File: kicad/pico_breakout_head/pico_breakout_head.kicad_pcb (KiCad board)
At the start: 2 copper layers, 39 x 66 mm, 19 parts, among them J1 HDR F 2.54MM 20-pin VERT, J2 HDR F 2.54MM 20-pin VERT, J3 JST B6B-PH-K-S, J4 HDR M 2.54MM 4p VERT, J5 JST B2B-XH-A, J6 HDR M 2.54MM 9p VERT, Q1 BSS123, U1 Pico

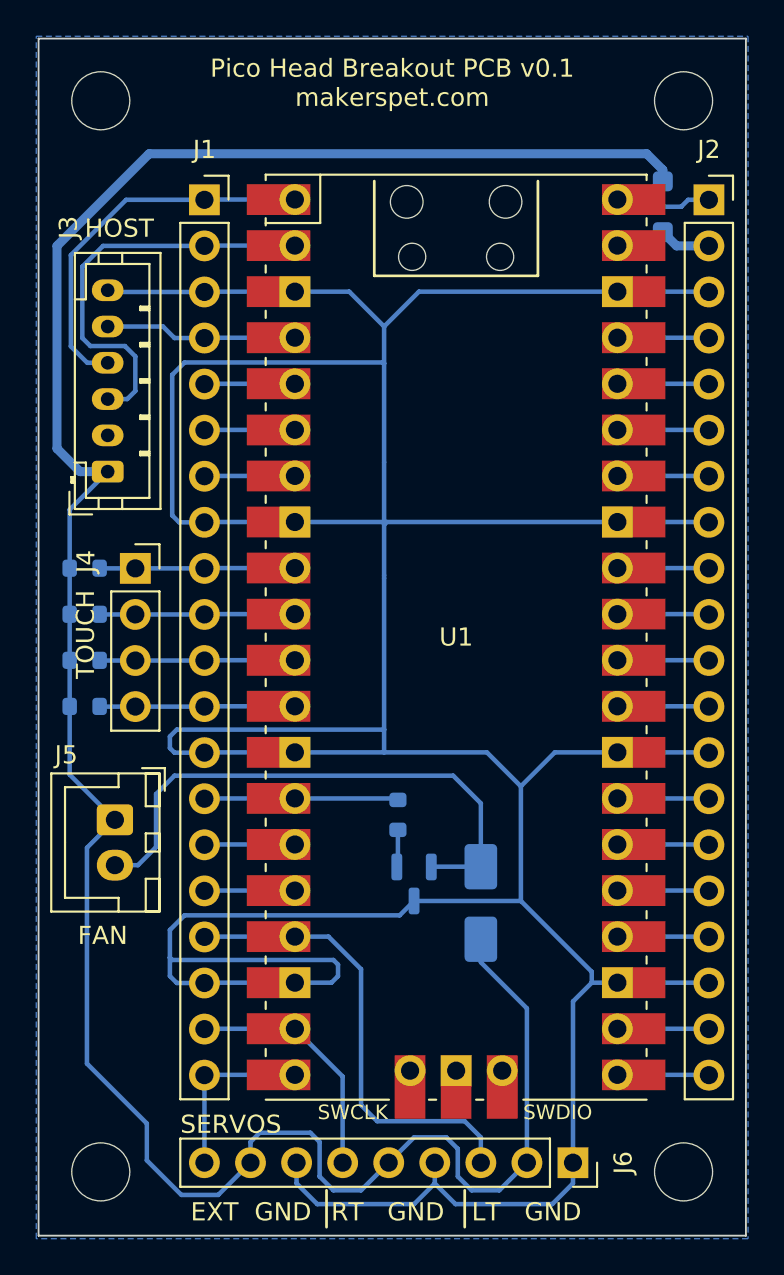
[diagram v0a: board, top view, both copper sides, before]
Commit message: Pico head PCB 0.1.1
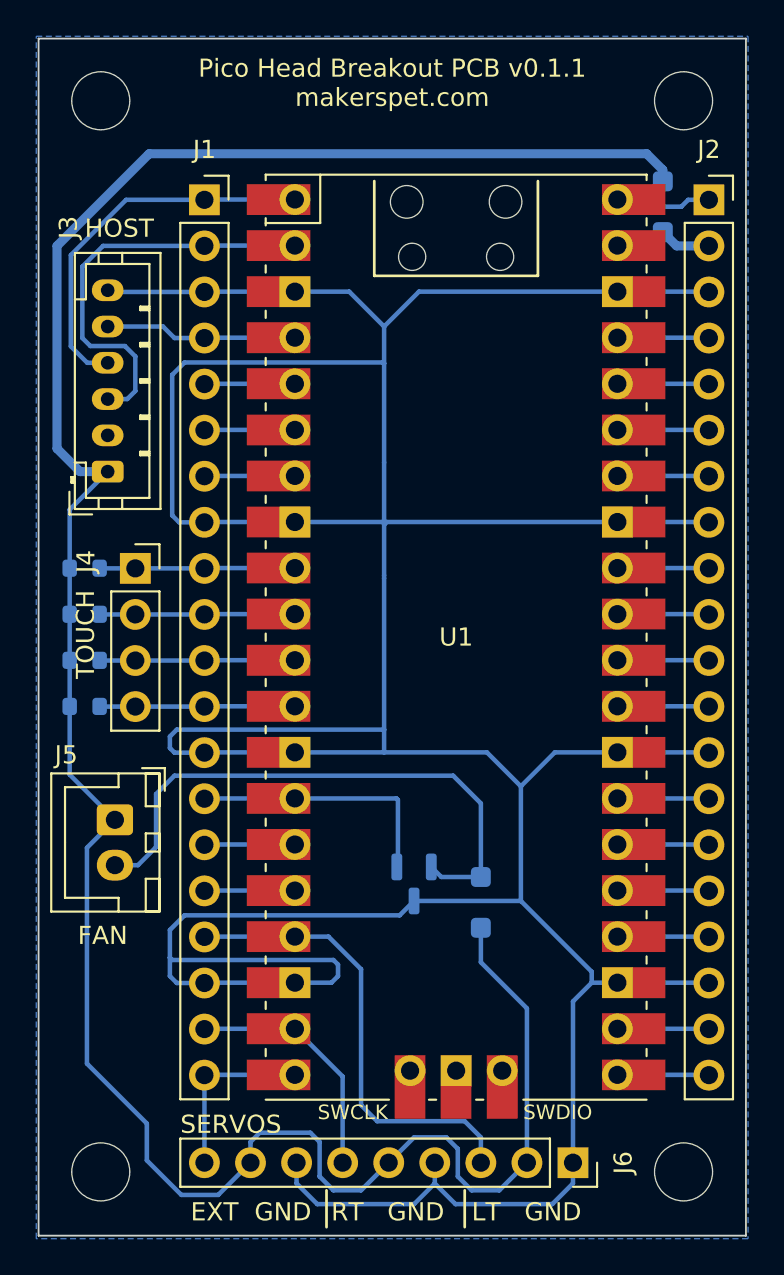
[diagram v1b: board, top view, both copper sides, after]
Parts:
- removed R5: 1k, Resistor_SMD:R_0603_1608Metric
- D1: value CGRA4004-G -> FS26; footprint Diode_SMD:D_SMA -> Diode_SMD:D_SOD-123F
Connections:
- Q1 pad 1: Net-(Q1-G) -> /FAN_EN
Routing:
- net /FAN_EN: track 10.7 -> 14.4 mm
- net Net-(Q1-G): track 2.07 -> 0.00 mm
- net Net-(D1-A): track 30.8 -> 31.6 mm
- net +5V: track 136.5 -> 137.1 mm
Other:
- board text added: "Pico Head Breakout PCB v0.1.1 makerspet.com"
- board text removed: "Pico Head Breakout PCB v0.1 makerspet.com"
